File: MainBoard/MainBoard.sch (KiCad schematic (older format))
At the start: 77 parts, among them IC1 MAX30102, IC2 TESEO-LIV3F, J1 USB_C_Receptacle_USB2.0, J2 Micro_SD_Card, J3 Conn_01x30_Female, Q1 DMG2301L, SW1 SW_DIP_x01, SW2 SW_DIP_x01, SW3 SW_DIP_x01, U1 MCP73831-2-OT, U2 MDBT50Q-1MV2, U3 LSM303C, U4 AP2112K-3.3, U5 VL53L1CXV0FY1, U6 MPL3115A2, U7 Si7050-A20, Y1 ABS05W

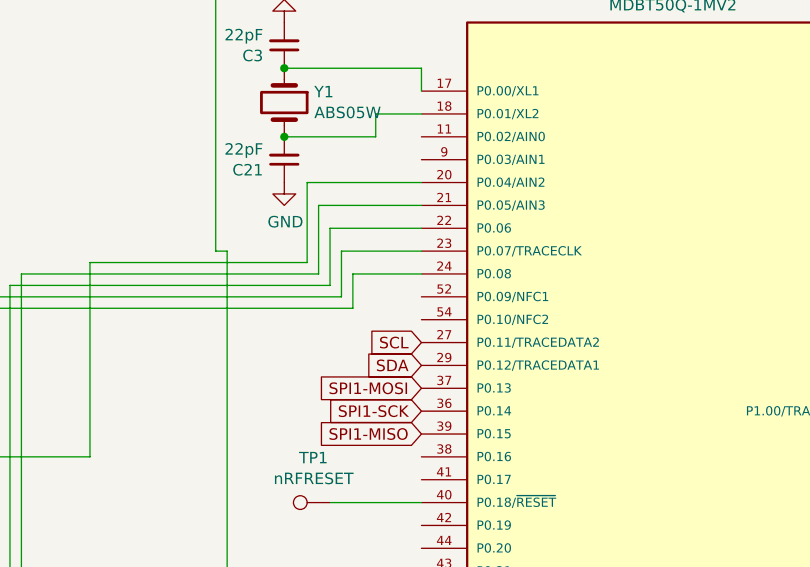
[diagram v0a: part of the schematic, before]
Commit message: route board
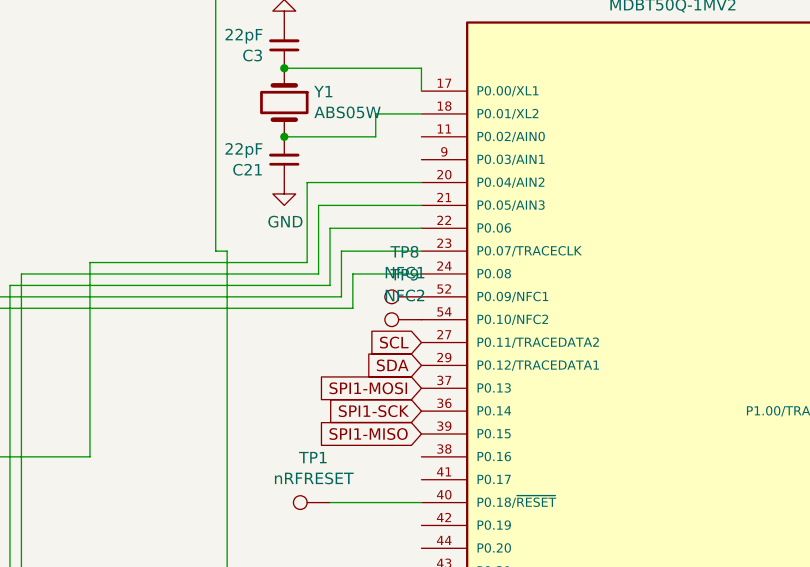
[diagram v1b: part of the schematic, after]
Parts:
- added TP8: NFC1, TestPoint:TestPoint_Pad_2.0x2.0mm, symbol MainBoard-rescue:TestPoint-Connector
- added TP9: NFC2, TestPoint:TestPoint_Pad_2.0x2.0mm, symbol MainBoard-rescue:TestPoint-Connector
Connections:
- net at U2.52 (P0.09/NFC1): now also TP8.1
- net at U2.54 (P0.10/NFC2): now also TP9.1
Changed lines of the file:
@@
 	0    1    1    0
 $EndComp
+$Comp
+L MainBoard-rescue:TestPoint-Connector TP8
+U 1 1 60BAC43F
+P 6600 6300
+F 0 "TP8" V 6795 6372 50  0000 C CNN
+F 1 "NFC1" V 6704 6372 50  0000 C CNN
+F 2 "TestPoint:TestPoint_Pad_2.0x2.0mm" H 6800 6300 50  0001 C CNN
+F 3 "~" H 6800 6300 50  0001 C CNN
+	1    6600 6300
+	0    -1   -1   0
+$EndComp
+$Comp
+L MainBoard-rescue:TestPoint-Connector TP9
+U 1 1 60BB7090
+P 6600 6400
+F 0 "TP9" V 6795 6472 50  0000 C CNN
+F 1 "NFC2" V 6704 6472 50  0000 C CNN
+F 2 "TestPoint:TestPoint_Pad_2.0x2.0mm" H 6800 6400 50  0001 C CNN
+F 3 "~" H 6800 6400 50  0001 C CNN
+	1    6600 6400
+	0    -1   -1   0
+$EndComp
 $EndSCHEMATC
